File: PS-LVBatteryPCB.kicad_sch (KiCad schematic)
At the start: 7 parts, among them J1 NTC_01_IN, J2 NTC_02_IN, J3 NTC_OUT, J4 BATT+, J6 BATT-, J7 SUPP-

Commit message: updated fps
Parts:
- F1: footprint Keystone 3568:FUSE_3568 -> Fuse:Fuseholder_Blade_Mini_Keystone_3568
- J6: footprint Keystone 3568:KEYSTONE_8191-6 -> UTSVT_Connectors:KEYSTONE_8191-SEMS
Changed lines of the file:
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@@
 			)
 		)
-		(property "Footprint" "Keystone 3568:FUSE_3568"
+		(property "Footprint" "Fuse:Fuseholder_Blade_Mini_Keystone_3568"
 			(at 133.35 80.01 0)
 			(effects
@@
 			)
 		)
-		(property "Footprint" "Keystone 3568:KEYSTONE_8191-6"
+		(property "Footprint" "UTSVT_Connectors:KEYSTONE_8191-SEMS"
 			(at 153.67 59.69 0)
 			(effects

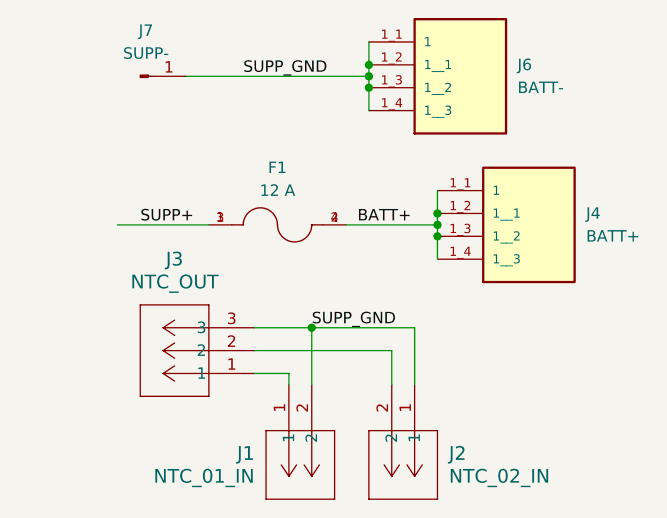
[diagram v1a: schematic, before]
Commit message: added footprints/layout
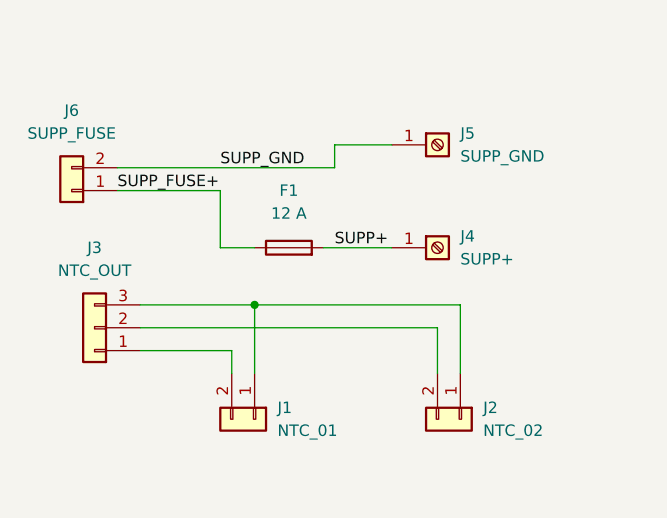
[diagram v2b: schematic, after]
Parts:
- removed F1: 12 A, Fuse:Fuseholder_Blade_Mini_Keystone_3568, symbol keystone 3568:3568
- removed J1: NTC_01_IN, Keystone 3568:CONN_SD-105313-100_02_MOL, symbol LHR:1053131102
- removed J2: NTC_02_IN, Keystone 3568:CONN_SD-105313-100_02_MOL, symbol LHR:1053131102
- removed J3: NTC_OUT, Keystone 3568:CONN_SD-105313-100_03_MOL, symbol LHR:1053131103
- removed J4: BATT+, Keystone 3568:KEYSTONE_8191-6, symbol LHR:8191-6
- removed J6: BATT-, UTSVT_Connectors:KEYSTONE_8191-SEMS, symbol LHR:8191-6
- removed J7: SUPP-, TestPoint:TestPoint_THTPad_2.0x2.0mm_Drill1.0mm, symbol Connector:Conn_01x01_Pin
- added F1: 12 A, Fuse:Fuseholder_Blade_Mini_Keystone_3568, symbol Device:Fuse
- added J1: NTC_01, UTSVT_Connectors:Molex_Nano-Fit_105309-xx02_1x02_P2.50mm_Vertical, symbol Connector_Generic:Conn_01x02
- added J2: NTC_02, UTSVT_Connectors:Molex_Nano-Fit_105309-xx02_1x02_P2.50mm_Vertical, symbol Connector_Generic:Conn_01x02
- added J3: NTC_OUT, Connector_Molex:Molex_Nano-Fit_105309-xx03_1x03_P2.50mm_Vertical, symbol Connector_Generic:Conn_01x03
- added J4: SUPP+, UTSVT_Connectors:KEYSTONE_8191-SEMS, symbol Connector:Screw_Terminal_01x01
- added J5: SUPP_GND, UTSVT_Connectors:KEYSTONE_8191-SEMS, symbol Connector:Screw_Terminal_01x01
- added J6: SUPP_FUSE, UTSVT_Connectors:AMASS_XT30PW-M_1x02_P2.50mm_Horizontal, symbol Connector_Generic:Conn_01x02
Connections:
- net SUPP+: now also F1.2, J4.1 (Pin_1)
- net SUPP_GND: now also J5.1 (Pin_1), J6.2 (Pin_2)
- new net: J1.1 (Pin_1), J2.1 (Pin_1), J3.3 (Pin_3)
- new net: J2.2 (Pin_2), J3.2 (Pin_2)
- new net: J1.2 (Pin_2), J3.1 (Pin_1)
- new net SUPP_FUSE+: F1.1, J6.1 (Pin_1)

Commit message: reorganized pcb and changed up fp's
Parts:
- J1, J2: footprint UTSVT_Connectors:Molex_Nano-Fit_105309-xx02_1x02_P2.50mm_Vertical -> Connector_Molex:Molex_Nano-Fit_105313-xx02_1x02_P2.50mm_Horizontal
- J6: footprint UTSVT_Connectors:AMASS_XT30PW-M_1x02_P2.50mm_Horizontal -> UTSVT_Connectors:AMASS_XT30UPB-M_1x02_P5.0mm_Vertical
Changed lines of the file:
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@@
 			)
 		)
-		(property "Footprint" "UTSVT_Connectors:Molex_Nano-Fit_105309-xx02_1x02_P2.50mm_Vertical"
+		(property "Footprint" "Connector_Molex:Molex_Nano-Fit_105313-xx02_1x02_P2.50mm_Horizontal"
 			(at 153.67 101.6 0)
 			(effects
@@
 			)
 		)
-		(property "Footprint" "UTSVT_Connectors:AMASS_XT30PW-M_1x02_P2.50mm_Horizontal"
+		(property "Footprint" "UTSVT_Connectors:AMASS_XT30UPB-M_1x02_P5.0mm_Vertical"
 			(at 110.49 76.2 0)
 			(effects
@@
 			)
 		)
-		(property "Footprint" "UTSVT_Connectors:Molex_Nano-Fit_105309-xx02_1x02_P2.50mm_Vertical"
+		(property "Footprint" "Connector_Molex:Molex_Nano-Fit_105313-xx02_1x02_P2.50mm_Horizontal"
 			(at 130.81 101.6 0)
 			(effects

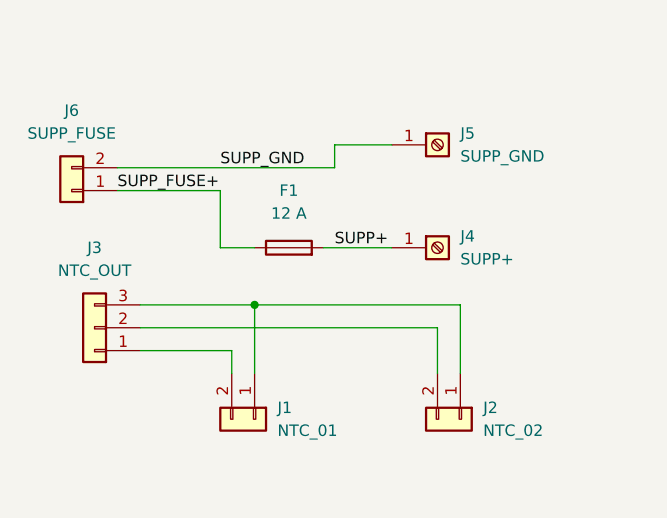
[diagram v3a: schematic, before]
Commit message: reorganize and added SOME 3D models
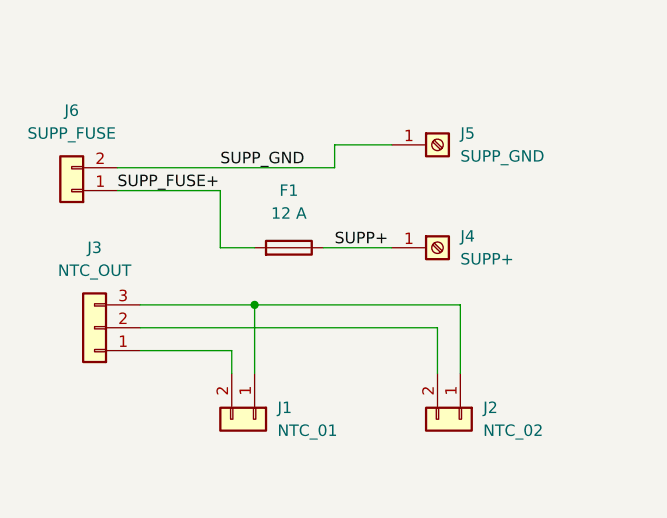
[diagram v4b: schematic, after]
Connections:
- net SUPP+: now also F1.1; no longer F1.2
- net SUPP_FUSE+: now also F1.2; no longer F1.1
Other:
- moved on the sheet: F1
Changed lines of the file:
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@@
 	(symbol
 		(lib_id "Device:Fuse")
-		(at 134.62 82.55 90)
+		(at 134.62 82.55 270)
+		(mirror x)
 		(unit 1)
 		(exclude_from_sim no)
